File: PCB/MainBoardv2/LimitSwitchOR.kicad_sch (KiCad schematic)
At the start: 3 parts, among them J6 Conn_01x03_Socket, U2 CD74HC00_N_14, U3 CD74HC00_N_14

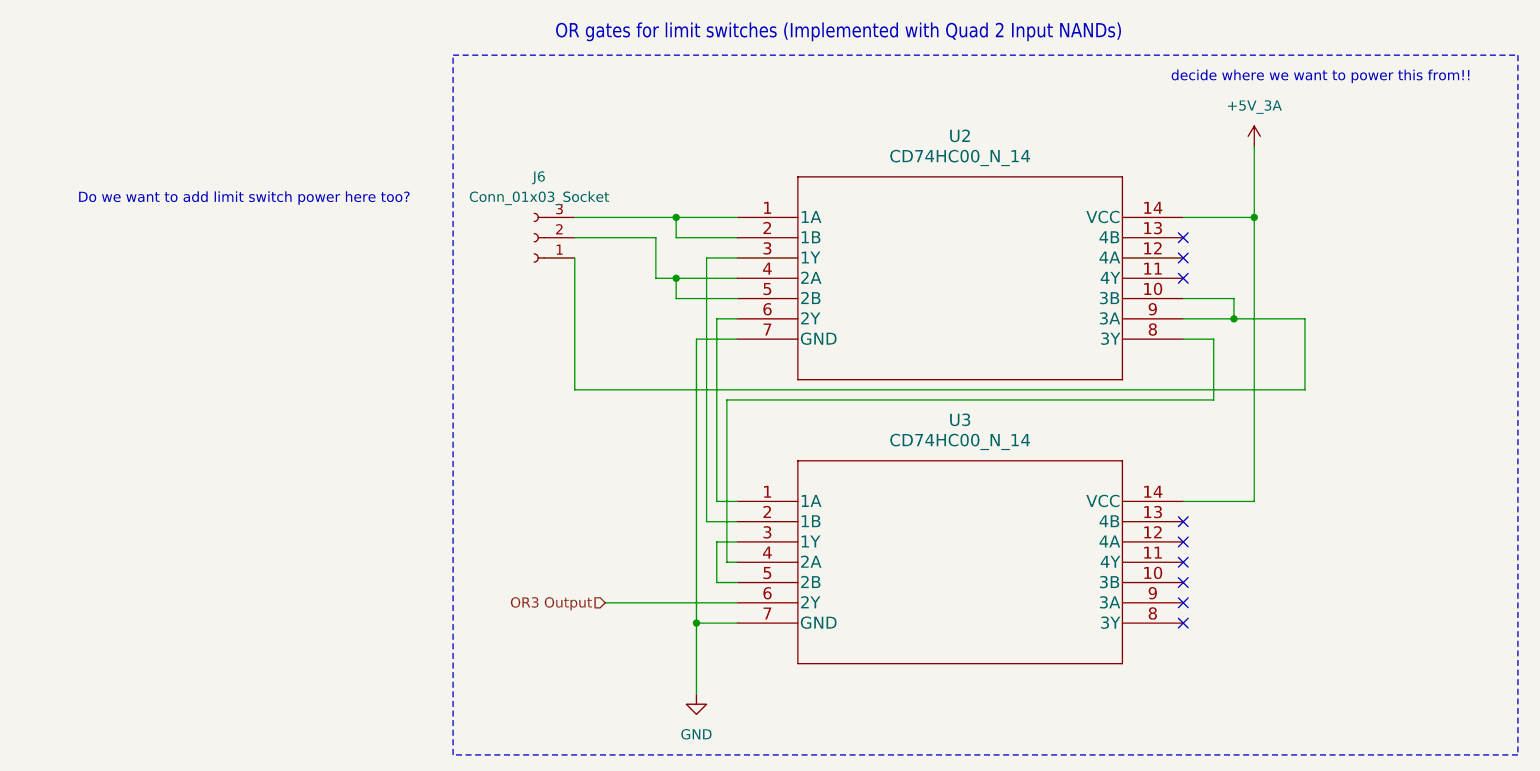
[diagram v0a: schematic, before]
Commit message: updating main board v2 progress
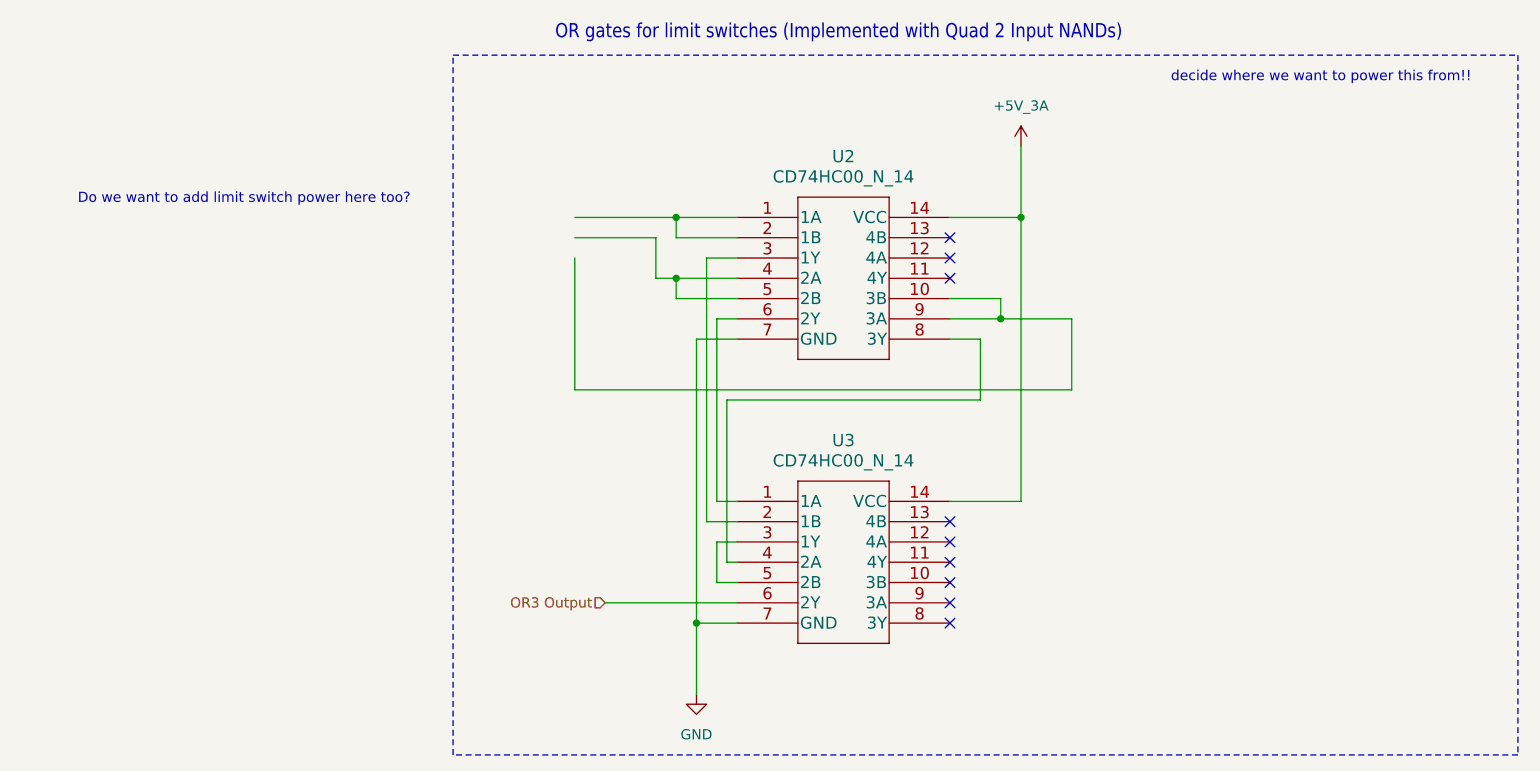
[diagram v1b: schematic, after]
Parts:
- removed J6: Conn_01x03_Socket, Connector_PinHeader_2.54mm:PinHeader_1x03_P2.54mm_Vertical, symbol Connector:Conn_01x03_Socket
- U2, U3: footprint Package_DIP:DIP-14_W7.62mm_LongPads -> N14
